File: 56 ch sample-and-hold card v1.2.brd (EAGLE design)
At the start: 221 x 38.7 mm, 144 parts, among them IC1 74HCT4051D, IC10 TL074JT, IC11 74HCT4051D, IC12 TL074JT, IC13 TL074JT, IC14 74HCT4051D, IC15 TL074JT, IC16 TL074JT, IC17 74HCT4051D, IC18 TL074JT, IC19 TL074JT, IC2 DAC8565F, IC20 74HCT4051D, IC21 TL074JT, IC22 TL074JT, IC26 74HCT4051D, IC27 TL074JT, IC28 TL074JT, IC3 TL074JT, IC5 78L05F, IC6 TL074JT, IC7 74HCT4051D, IC8 TL074JT, IC9 TL074JT, X10 MA07-2J-FEMALE, X4 DNM, X5 DNM, X6 MA08-2J-FEMALE, X9 DNM

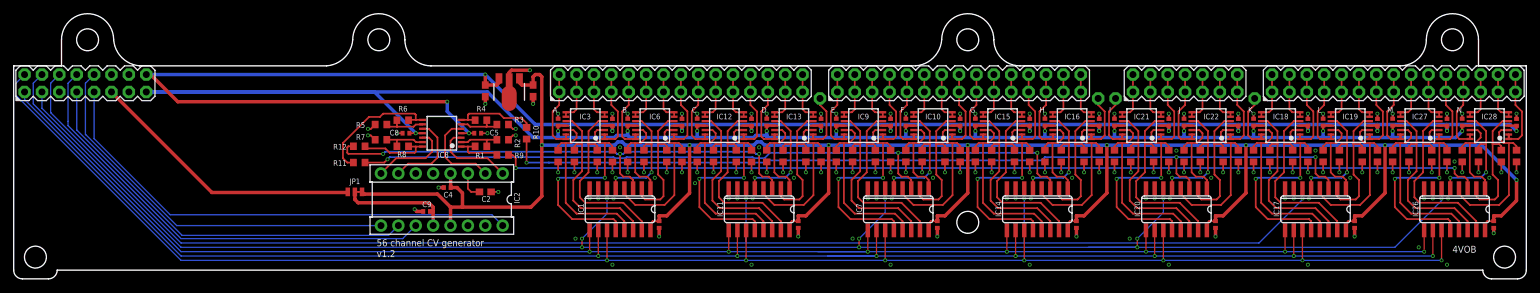
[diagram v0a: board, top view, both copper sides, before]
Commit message: DRC ok
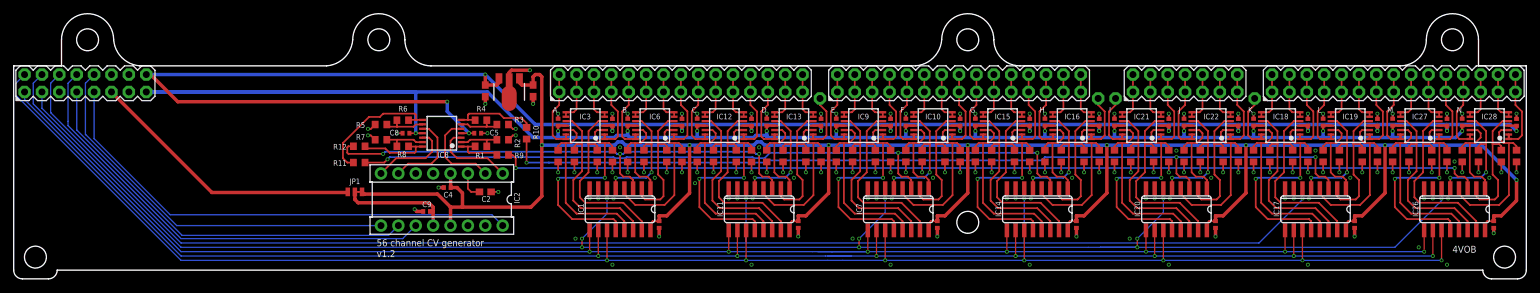
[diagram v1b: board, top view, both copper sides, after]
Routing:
- net A1: track 249.7 -> 246.1 mm
- net -12V: track 278.7 -> 282.2 mm
- net INH_0: track 257.8 -> 256.0 mm
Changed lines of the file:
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@@
 <layer number="17" name="Pads" color="2" fill="1" visible="yes" active="yes"/>
 <layer number="18" name="Vias" color="2" fill="1" visible="yes" active="yes"/>
-<layer number="19" name="Unrouted" color="6" fill="1" visible="yes" active="yes"/>
+<layer number="19" name="Unrouted" color="6" fill="1" visible="no" active="yes"/>
 <layer number="20" name="Dimension" color="15" fill="1" visible="yes" active="yes"/>
 <layer number="21" name="tPlace" color="7" fill="1" visible="yes" active="yes"/>
@@
 <via x="56.03875" y="20.0025" extent="1-16" drill="0.3302"/>
 <polygon width="0.127" layer="2">
-<vertex x="41.275" y="40.005"/>
+<vertex x="-1.11125" y="40.005"/>
 <vertex x="222.25" y="40.005"/>
 <vertex x="222.25" y="-1.27"/>
-<vertex x="41.275" y="-1.27"/>
+<vertex x="-1.11125" y="-1.27"/>
 </polygon>
 <polygon width="0.127" layer="15">
-<vertex x="40.005" y="41.275"/>
+<vertex x="-1.905" y="41.275"/>
 <vertex x="223.52" y="41.275"/>
 <vertex x="223.52" y="-1.905"/>
-<vertex x="40.005" y="-1.905"/>
+<vertex x="-1.905" y="-1.905"/>
 </polygon>
 <wire x1="72.39" y1="27.762" x2="72.39" y2="25.095" width="0.254" layer="1"/>
 <contactref element="X6" pad="14"/>
-<wire x1="51.7525" y1="20.6375" x2="16.8275" y2="28.575" width="0" layer="19" extent="1-1"/>
 </signal>
 <signal name="OUT_0">
@@
 <wire x1="110.1725" y1="19.3675" x2="110.01375" y2="19.52625" width="0.508" layer="16"/>
 <wire x1="120.17375" y1="19.3675" x2="110.1725" y2="19.3675" width="0.508" layer="16"/>
-<wire x1="58.7375" y1="20.0025" x2="52.705" y2="26.035" width="0.508" layer="16"/>
-<wire x1="52.705" y1="26.035" x2="19.3675" y2="26.035" width="0.508" layer="16"/>
+<wire x1="58.7375" y1="20.0025" x2="58.7375" y2="26.035" width="0.508" layer="16"/>
+<wire x1="58.7375" y1="26.035" x2="19.3675" y2="26.035" width="0.508" layer="16"/>
 </signal>
 <signal name="OUT_7">
@@
 <via x="208.5975" y="1.42875" extent="1-16" drill="0.3302"/>
 <wire x1="86.6775" y1="1.42875" x2="106.9975" y2="1.42875" width="0.13" layer="16"/>
-<wire x1="106.9975" y1="1.42875" x2="127.3175" y2="1.42875" width="0.13" layer="16"/>
+<wire x1="106.9975" y1="1.42875" x2="118.90375" y2="1.42875" width="0.13" layer="16"/>
+<wire x1="121.12625" y1="1.42875" x2="127.3175" y2="1.42875" width="0.13" layer="16"/>
 <wire x1="127.3175" y1="1.42875" x2="147.6375" y2="1.42875" width="0.13" layer="16"/>
 <wire x1="147.6375" y1="1.42875" x2="167.9575" y2="1.42875" width="0.13" layer="16"/>
@@
 <wire x1="0.3175" y1="27.305" x2="1.5875" y2="28.575" width="0.127" layer="16"/>
 <wire x1="0.3175" y1="25.55875" x2="0.3175" y2="27.305" width="0.127" layer="16"/>
+<wire x1="118.90375" y1="1.42875" x2="121.12625" y2="1.42875" width="0.127" layer="16"/>
 </signal>
 <signal name="A1">
@@
 <wire x1="187.0075" y1="2.06375" x2="166.6875" y2="2.06375" width="0.13" layer="16"/>
 <wire x1="166.6875" y1="2.06375" x2="146.3675" y2="2.06375" width="0.13" layer="16"/>
-<wire x1="146.3675" y1="2.06375" x2="118.90375" y2="2.06375" width="0.13" layer="16"/>
-<wire x1="126.0475" y1="2.06375" x2="105.7275" y2="2.06375" width="0.13" layer="16"/>
+<wire x1="146.3675" y1="2.06375" x2="126.0475" y2="2.06375" width="0.13" layer="16"/>
+<wire x1="122.39625" y1="2.06375" x2="118.90375" y2="2.06375" width="0.13" layer="16"/>
+<wire x1="126.0475" y1="2.06375" x2="122.39625" y2="2.06375" width="0.13" layer="16"/>
+<wire x1="105.7275" y1="2.06375" x2="118.58625" y2="2.06375" width="0.13" layer="16"/>
 <wire x1="105.7275" y1="2.06375" x2="85.4075" y2="2.06375" width="0.13" layer="16"/>
 <wire x1="85.4075" y1="2.06375" x2="85.4075" y2="5.8166" width="0.13" layer="1"/>
@@
 <wire x1="85.4075" y1="2.06375" x2="24.4475" y2="2.06375" width="0.13" layer="16"/>
 <contactref element="X6" pad="1"/>
-<wire x1="126.0475" y1="2.06375" x2="118.90375" y2="2.06375" width="0" layer="19" extent="16-16"/>
+<wire x1="118.58625" y1="2.06375" x2="122.39625" y2="2.06375" width="0.127" layer="16"/>
 </signal>
 <signal name="A2">
@@
 <wire x1="185.7375" y1="2.69875" x2="165.4175" y2="2.69875" width="0.13" layer="16"/>
 <wire x1="165.4175" y1="2.69875" x2="145.0975" y2="2.69875" width="0.13" layer="16"/>
-<wire x1="145.0975" y1="2.69875" x2="117.475" y2="2.69875" width="0.13" layer="16"/>
-<wire x1="124.7775" y1="2.69875" x2="104.4575" y2="2.69875" width="0.13" layer="16"/>
+<wire x1="145.0975" y1="2.69875" x2="119.53875" y2="2.69875" width="0.13" layer="16"/>
+<wire x1="119.53875" y1="2.69875" x2="117.475" y2="2.69875" width="0.13" layer="16"/>
+<wire x1="104.4575" y1="2.69875" x2="116.68125" y2="2.69875" width="0.13" layer="16"/>
 <wire x1="104.4575" y1="2.69875" x2="84.1375" y2="2.69875" width="0.13" layer="16"/>
 <wire x1="84.1375" y1="5.8166" x2="84.1375" y2="2.69875" width="0.13" layer="1"/>
@@
 <wire x1="2.8575" y1="27.305" x2="4.1275" y2="28.575" width="0.13" layer="16"/>
 <wire x1="2.8575" y1="24.28875" x2="2.8575" y2="27.305" width="0.13" layer="16"/>
-<wire x1="124.7775" y1="2.69875" x2="117.475" y2="2.69875" width="0" layer="19" extent="16-16"/>
+<wire x1="124.7775" y1="2.69875" x2="119.53875" y2="2.69875" width="0.127" layer="16"/>
+<wire x1="116.68125" y1="2.69875" x2="119.53875" y2="2.69875" width="0.127" layer="16"/>
 </signal>
 <signal name="INH_0">
@@
 <wire x1="208.5975" y1="10.16" x2="201.77125" y2="3.33375" width="0.13" layer="16"/>
 <wire x1="83.02625" y1="4.60375" x2="83.02625" y2="3.33375" width="0.13" layer="1"/>
-<wire x1="201.77125" y1="3.33375" x2="157.00375" y2="3.33375" width="0.13" layer="16"/>
-<wire x1="164.1475" y1="3.33375" x2="123.5075" y2="3.33375" width="0.13" layer="16"/>
+<wire x1="201.77125" y1="3.33375" x2="158.75" y2="3.33375" width="0.13" layer="16"/>
+<wire x1="158.75" y1="3.33375" x2="157.00375" y2="3.33375" width="0.13" layer="16"/>
+<wire x1="157.00375" y1="3.33375" x2="123.5075" y2="3.33375" width="0.13" layer="16"/>
 <wire x1="123.5075" y1="3.33375" x2="83.02625" y2="3.33375" width="0.13" layer="16"/>
 <via x="83.02625" y="3.33375" extent="1-16" drill="0.3302"/>
@@
 <wire x1="4.1275" y1="25.87625" x2="4.1275" y2="26.035" width="0.13" layer="16"/>
 <wire x1="4.1275" y1="23.65375" x2="4.1275" y2="26.035" width="0.127" layer="16"/>
-<wire x1="164.1475" y1="3.33375" x2="157.00375" y2="3.33375" width="0" layer="19" extent="16-16"/>
+<wire x1="164.1475" y1="3.33375" x2="158.75" y2="3.33375" width="0.127" layer="16"/>
 </signal>
 <signal name="DAC_1">
@@
 <mfgpreviewcolor name="substratecolor" color="0xFF786E46"/>
 </mfgpreviewcolors>
-<errors>
-</errors>
 </board>
 </drawing>
